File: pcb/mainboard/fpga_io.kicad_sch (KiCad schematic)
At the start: 18 parts, among them SW3 DSHP02TS, U3 XC7Z010-CLG400

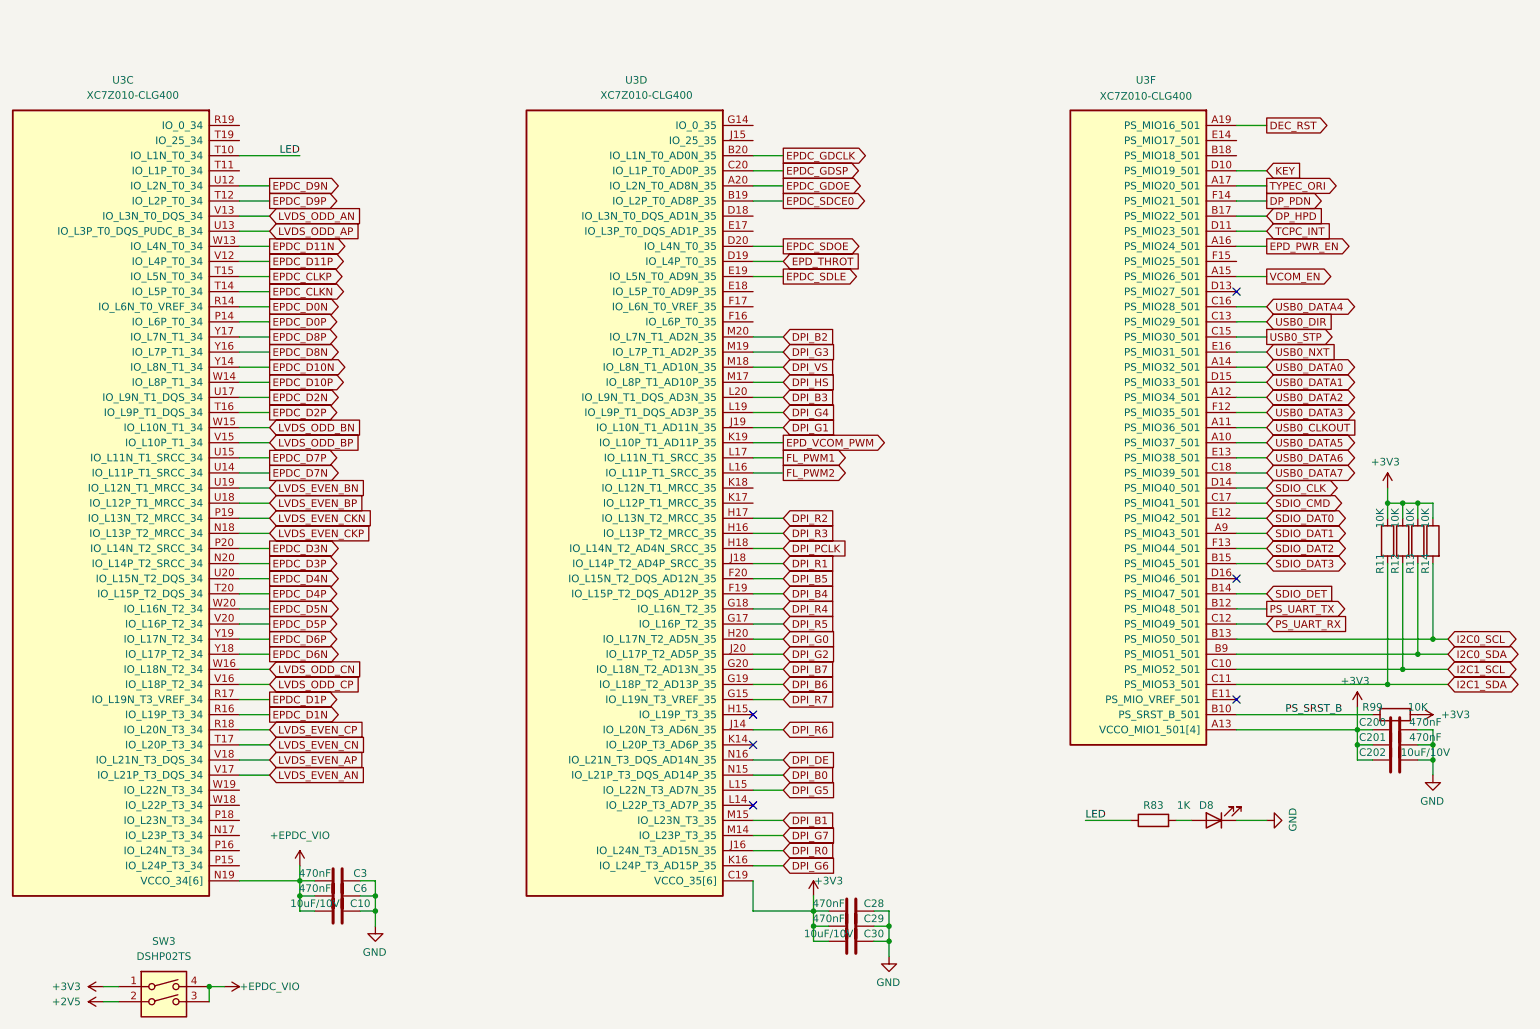
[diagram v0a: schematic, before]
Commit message: PCB r0p10 wip
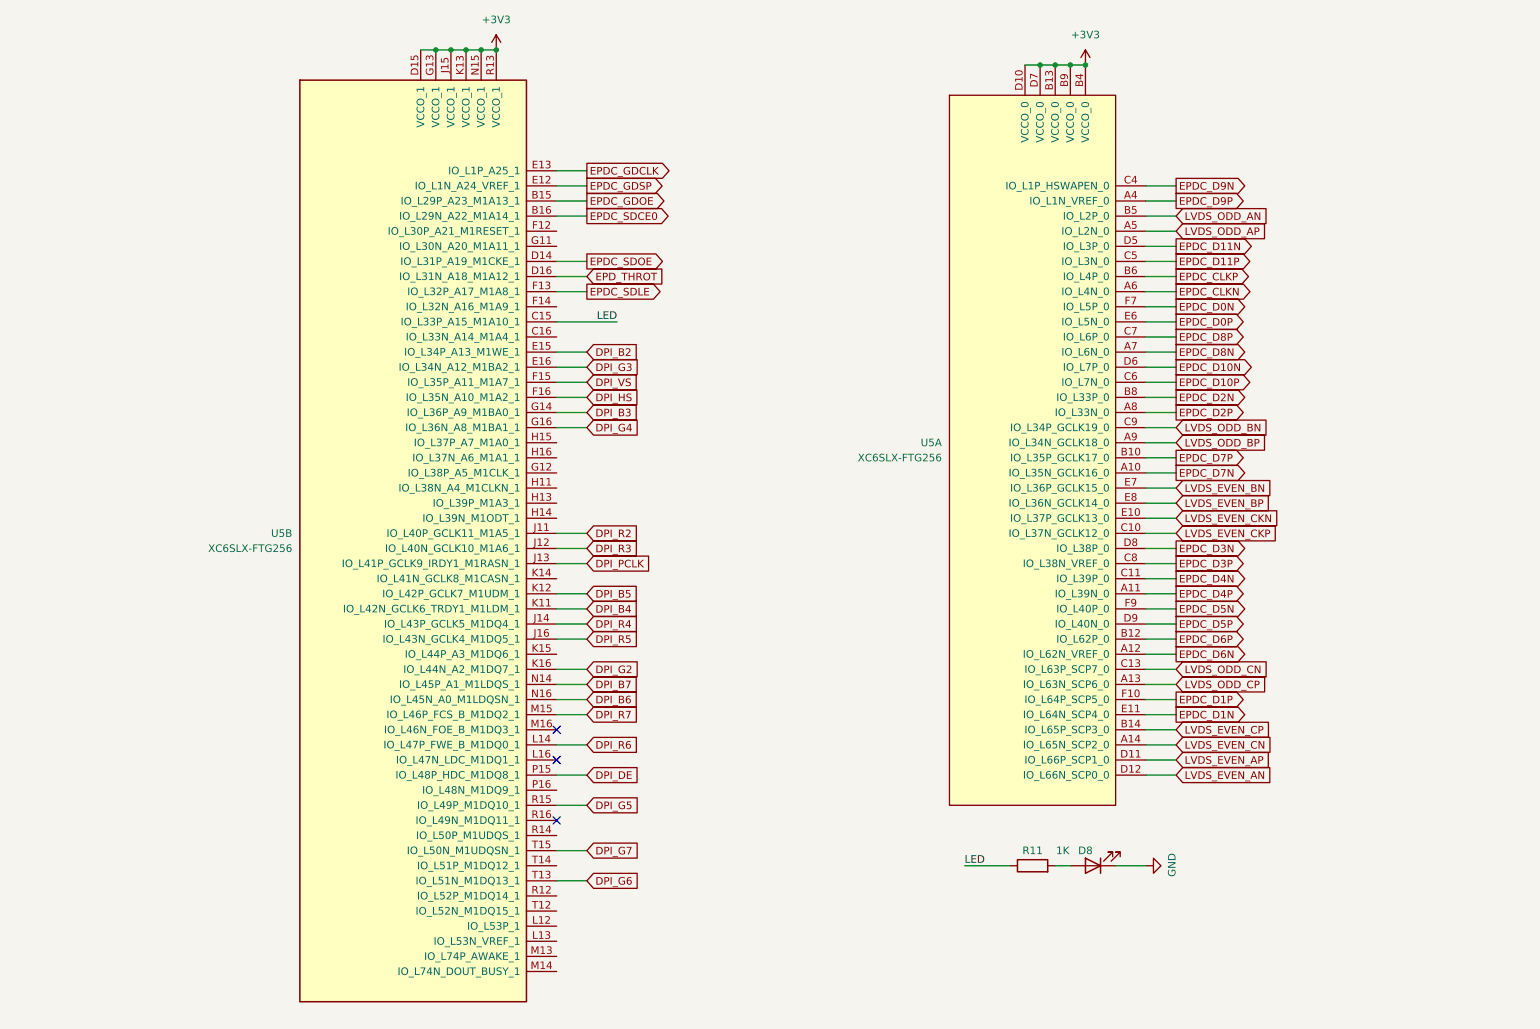
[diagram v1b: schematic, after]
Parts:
- removed C10, C202, C30: 10uF/10V, Capacitor_SMD:C_0603_1608Metric, symbol Device:C
- removed C200, C201, C28, C29, C3, C6: 470nF, Capacitor_SMD:C_0402_1005Metric, symbol Device:C
- removed R12, R13, R14, R99: 10K, Resistor_SMD:R_0402_1005Metric, symbol Device:R
- removed R83: 1K, Resistor_SMD:R_0402_1005Metric, symbol Device:R
- removed SW3: DSHP02TS, Button_Switch_SMD:SW_DIP_SPSTx02_Slide_KingTek_DSHP02TS_W7.62mm_P1.27mm, symbol Switch:SW_DIP_x02
- removed U3: XC7Z010-CLG400, Package_BGA:Xilinx_CLG400, symbol symbols:XC7Z007S-CLG400
- added U5: XC6SLX-FTG256, symbol symbols:XC6SLX-FTG256
- R11: value 10K -> 1K
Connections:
- net I2C1_SDA is gone; now on an unnamed net: R11.2
- net +3V3: now also U5.B13 (VCCO_0), U5.B4 (VCCO_0), U5.B9 (VCCO_0), U5.D10 (VCCO_0), U5.D15 (VCCO_1), U5.D7 (VCCO_0), U5.G13 (VCCO_1), U5.J15 (VCCO_1), U5.K13 (VCCO_1), U5.N15 (VCCO_1), U5.R13 (VCCO_1); no longer R11.1
- net DPI_B2: now also U5.E15 (IO_L34P_A13_M1WE_1)
- net DPI_B3: now also U5.G14 (IO_L36P_A9_M1BA0_1)
- net DPI_B4: now also U5.K11 (IO_L42N_GCLK6_TRDY1_M1LDM_1)
- net DPI_B5: now also U5.K12 (IO_L42P_GCLK7_M1UDM_1)
- net DPI_B6: now also U5.N16 (IO_L45N_A0_M1LDQSN_1)
- net DPI_B7: now also U5.N14 (IO_L45P_A1_M1LDQS_1)
- net DPI_DE: now also U5.P15 (IO_L48P_HDC_M1DQ8_1)
- net DPI_G2: now also U5.K16 (IO_L44N_A2_M1DQ7_1)
- net DPI_G3: now also U5.E16 (IO_L34N_A12_M1BA2_1)
- net DPI_G4: now also U5.G16 (IO_L36N_A8_M1BA1_1)
- net DPI_G5: now also U5.R15 (IO_L49P_M1DQ10_1)
- net DPI_G6: now also U5.T13 (IO_L51N_M1DQ13_1)
- net DPI_G7: now also U5.T15 (IO_L50N_M1UDQSN_1)
- net DPI_HS: now also U5.F16 (IO_L35N_A10_M1A2_1)
- net DPI_PCLK: now also U5.J13 (IO_L41P_GCLK9_IRDY1_M1RASN_1)
- net DPI_R2: now also U5.J11 (IO_L40P_GCLK11_M1A5_1)
- net DPI_R3: now also U5.J12 (IO_L40N_GCLK10_M1A6_1)
- net DPI_R4: now also U5.J14 (IO_L43P_GCLK5_M1DQ4_1)
- net DPI_R5: now also U5.J16 (IO_L43N_GCLK4_M1DQ5_1)
- net DPI_R6: now also U5.L14 (IO_L47P_FWE_B_M1DQ0_1)
- net DPI_R7: now also U5.M15 (IO_L46P_FCS_B_M1DQ2_1)
- net DPI_VS: now also U5.F15 (IO_L35P_A11_M1A7_1)
- net EPDC_CLKN: now also U5.A6 (IO_L4N_0)
- net EPDC_CLKP: now also U5.B6 (IO_L4P_0)
- net EPDC_D0N: now also U5.F7 (IO_L5P_0)
- net EPDC_D0P: now also U5.E6 (IO_L5N_0)
- net EPDC_D10N: now also U5.D6 (IO_L7P_0)
- net EPDC_D10P: now also U5.C6 (IO_L7N_0)
- net EPDC_D11N: now also U5.D5 (IO_L3P_0)
- net EPDC_D11P: now also U5.C5 (IO_L3N_0)
- net EPDC_D1N: now also U5.E11 (IO_L64N_SCP4_0)
- net EPDC_D1P: now also U5.F10 (IO_L64P_SCP5_0)
- net EPDC_D2N: now also U5.B8 (IO_L33P_0)
- net EPDC_D2P: now also U5.A8 (IO_L33N_0)
- net EPDC_D3N: now also U5.D8 (IO_L38P_0)
- net EPDC_D3P: now also U5.C8 (IO_L38N_VREF_0)
- net EPDC_D4N: now also U5.C11 (IO_L39P_0)
- net EPDC_D4P: now also U5.A11 (IO_L39N_0)
- net EPDC_D5N: now also U5.F9 (IO_L40P_0)
- net EPDC_D5P: now also U5.D9 (IO_L40N_0)
- net EPDC_D6N: now also U5.A12 (IO_L62N_VREF_0)
- net EPDC_D6P: now also U5.B12 (IO_L62P_0)
- net EPDC_D7N: now also U5.A10 (IO_L35N_GCLK16_0)
- net EPDC_D7P: now also U5.B10 (IO_L35P_GCLK17_0)
- net EPDC_D8N: now also U5.A7 (IO_L6N_0)
- net EPDC_D8P: now also U5.C7 (IO_L6P_0)
- net EPDC_D9N: now also U5.C4 (IO_L1P_HSWAPEN_0)
- net EPDC_D9P: now also U5.A4 (IO_L1N_VREF_0)
- net EPDC_GDCLK: now also U5.E13 (IO_L1P_A25_1)
- net EPDC_GDOE: now also U5.B15 (IO_L29P_A23_M1A13_1)
- net EPDC_GDSP: now also U5.E12 (IO_L1N_A24_VREF_1)
- net EPDC_SDCE0: now also U5.B16 (IO_L29N_A22_M1A14_1)
- net EPDC_SDLE: now also U5.F13 (IO_L32P_A17_M1A8_1)
- net EPDC_SDOE: now also U5.D14 (IO_L31P_A19_M1CKE_1)
- net EPD_THROT: now also U5.D16 (IO_L31N_A18_M1A12_1)
- net LED: now also R11.1, U5.C15 (IO_L33P_A15_M1A10_1)
- net LVDS_EVEN_AN: now also U5.D12 (IO_L66N_SCP0_0)
- net LVDS_EVEN_AP: now also U5.D11 (IO_L66P_SCP1_0)
- net LVDS_EVEN_BN: now also U5.E7 (IO_L36P_GCLK15_0)
- net LVDS_EVEN_BP: now also U5.E8 (IO_L36N_GCLK14_0)
- net LVDS_EVEN_CKN: now also U5.E10 (IO_L37P_GCLK13_0)
- net LVDS_EVEN_CKP: now also U5.C10 (IO_L37N_GCLK12_0)
- net LVDS_EVEN_CN: now also U5.A14 (IO_L65N_SCP2_0)
- net LVDS_EVEN_CP: now also U5.B14 (IO_L65P_SCP3_0)
- net LVDS_ODD_AN: now also U5.B5 (IO_L2P_0)
- net LVDS_ODD_AP: now also U5.A5 (IO_L2N_0)
- net LVDS_ODD_BN: now also U5.C9 (IO_L34P_GCLK19_0)
- net LVDS_ODD_BP: now also U5.A9 (IO_L34N_GCLK18_0)
- net LVDS_ODD_CN: now also U5.C13 (IO_L63P_SCP7_0)
- net LVDS_ODD_CP: now also U5.A13 (IO_L63N_SCP6_0)
- no-connect marks 6 -> 3

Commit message: PCB r0p10
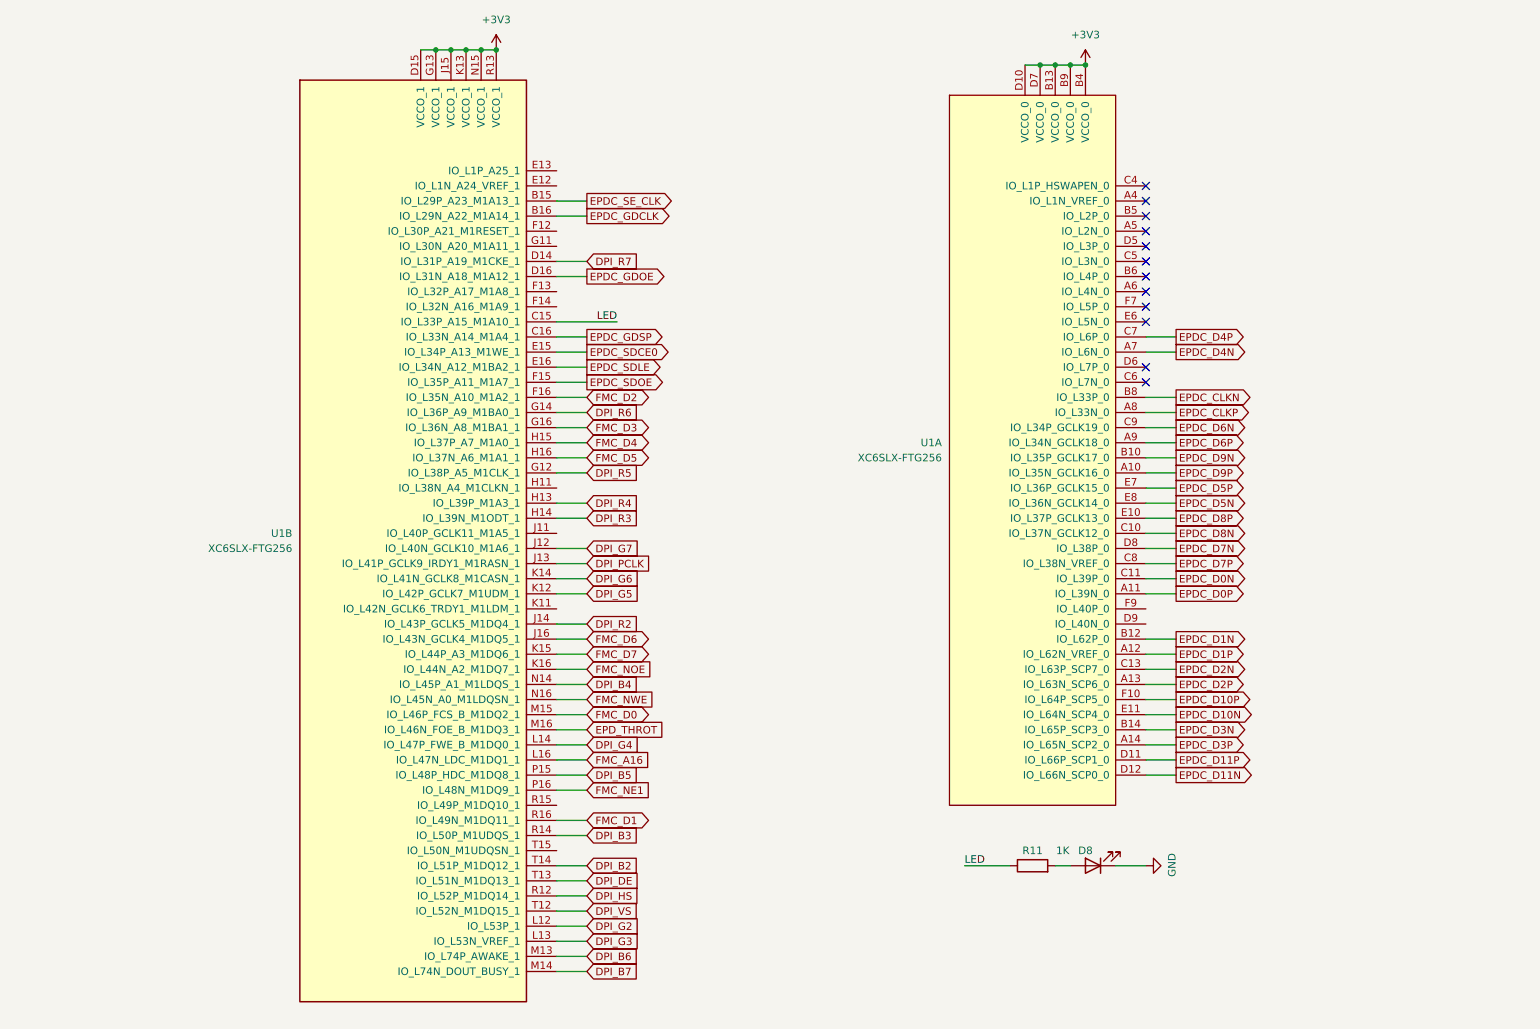
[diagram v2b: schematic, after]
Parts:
- U1: renamed from U5; footprint (none) -> footprints:Xilinx_FTG256
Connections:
- net LVDS_EVEN_AN is gone; now on net EPDC_D11N: U1.D12 (IO_L66N_SCP0_0)
- net LVDS_EVEN_AP is gone; now on net EPDC_D11P: U1.D11 (IO_L66P_SCP1_0)
- net LVDS_EVEN_BN is gone; now on net EPDC_D5P: U1.E7 (IO_L36P_GCLK15_0)
- net LVDS_EVEN_BP is gone; now on net EPDC_D5N: U1.E8 (IO_L36N_GCLK14_0)
- net LVDS_EVEN_CKN is gone; now on net EPDC_D8P: U1.E10 (IO_L37P_GCLK13_0)
- net LVDS_EVEN_CKP is gone; now on net EPDC_D8N: U1.C10 (IO_L37N_GCLK12_0)
- net LVDS_EVEN_CN is gone; now on net EPDC_D3P: U1.A14 (IO_L65N_SCP2_0)
- net LVDS_EVEN_CP is gone; now on net EPDC_D3N: U1.B14 (IO_L65P_SCP3_0)
- net LVDS_ODD_BN is gone; now on net EPDC_D6N: U1.C9 (IO_L34P_GCLK19_0)
- net LVDS_ODD_BP is gone; now on net EPDC_D6P: U1.A9 (IO_L34N_GCLK18_0)
- net LVDS_ODD_CN is gone; now on net EPDC_D2N: U1.C13 (IO_L63P_SCP7_0)
- net LVDS_ODD_CP is gone; now on net EPDC_D2P: U1.A13 (IO_L63N_SCP6_0)
- net DPI_B2: now also U1.T14 (IO_L51P_M1DQ12_1); no longer U1.E15 (IO_L34P_A13_M1WE_1)
- net DPI_B3: now also U1.R14 (IO_L50P_M1UDQS_1); no longer U1.G14 (IO_L36P_A9_M1BA0_1)
- net DPI_B4: now also U1.N14 (IO_L45P_A1_M1LDQS_1); no longer U1.K11 (IO_L42N_GCLK6_TRDY1_M1LDM_1)
- net DPI_B5: now also U1.P15 (IO_L48P_HDC_M1DQ8_1); no longer U1.K12 (IO_L42P_GCLK7_M1UDM_1)
- net DPI_B6: now also U1.M13 (IO_L74P_AWAKE_1); no longer U1.N16 (IO_L45N_A0_M1LDQSN_1)
- net DPI_B7: now also U1.M14 (IO_L74N_DOUT_BUSY_1); no longer U1.N14 (IO_L45P_A1_M1LDQS_1)
- net DPI_DE: now also U1.T13 (IO_L51N_M1DQ13_1); no longer U1.P15 (IO_L48P_HDC_M1DQ8_1)
- net DPI_G2: now also U1.L12 (IO_L53P_1); no longer U1.K16 (IO_L44N_A2_M1DQ7_1)
- net DPI_G3: now also U1.L13 (IO_L53N_VREF_1); no longer U1.E16 (IO_L34N_A12_M1BA2_1)
- net DPI_G4: now also U1.L14 (IO_L47P_FWE_B_M1DQ0_1); no longer U1.G16 (IO_L36N_A8_M1BA1_1)
- net DPI_G5: now also U1.K12 (IO_L42P_GCLK7_M1UDM_1); no longer U1.R15 (IO_L49P_M1DQ10_1)
- net DPI_G6: now also U1.K14 (IO_L41N_GCLK8_M1CASN_1); no longer U1.T13 (IO_L51N_M1DQ13_1)
- net DPI_G7: now also U1.J12 (IO_L40N_GCLK10_M1A6_1); no longer U1.T15 (IO_L50N_M1UDQSN_1)
- net DPI_HS: now also U1.R12 (IO_L52P_M1DQ14_1); no longer U1.F16 (IO_L35N_A10_M1A2_1)
- net DPI_R2: now also U1.J14 (IO_L43P_GCLK5_M1DQ4_1); no longer U1.J11 (IO_L40P_GCLK11_M1A5_1)
- net DPI_R3: now also U1.H14 (IO_L39N_M1ODT_1); no longer U1.J12 (IO_L40N_GCLK10_M1A6_1)
- net DPI_R4: now also U1.H13 (IO_L39P_M1A3_1); no longer U1.J14 (IO_L43P_GCLK5_M1DQ4_1)
- net DPI_R5: now also U1.G12 (IO_L38P_A5_M1CLK_1); no longer U1.J16 (IO_L43N_GCLK4_M1DQ5_1)
- net DPI_R6: now also U1.G14 (IO_L36P_A9_M1BA0_1); no longer U1.L14 (IO_L47P_FWE_B_M1DQ0_1)
- net DPI_R7: now also U1.D14 (IO_L31P_A19_M1CKE_1); no longer U1.M15 (IO_L46P_FCS_B_M1DQ2_1)
- net DPI_VS: now also U1.T12 (IO_L52N_M1DQ15_1); no longer U1.F15 (IO_L35P_A11_M1A7_1)
- net EPDC_CLKN: now also U1.B8 (IO_L33P_0); no longer U1.A6 (IO_L4N_0)
- net EPDC_CLKP: now also U1.A8 (IO_L33N_0); no longer U1.B6 (IO_L4P_0)
- net EPDC_D0N: now also U1.C11 (IO_L39P_0); no longer U1.F7 (IO_L5P_0)
- net EPDC_D0P: now also U1.A11 (IO_L39N_0); no longer U1.E6 (IO_L5N_0)
- net EPDC_D10N: now also U1.E11 (IO_L64N_SCP4_0); no longer U1.D6 (IO_L7P_0)
- net EPDC_D10P: now also U1.F10 (IO_L64P_SCP5_0); no longer U1.C6 (IO_L7N_0)
- net EPDC_D11N: no longer U1.D5 (IO_L3P_0)
- net EPDC_D11P: no longer U1.C5 (IO_L3N_0)
- net EPDC_D1N: now also U1.B12 (IO_L62P_0); no longer U1.E11 (IO_L64N_SCP4_0)
- net EPDC_D1P: now also U1.A12 (IO_L62N_VREF_0); no longer U1.F10 (IO_L64P_SCP5_0)
- net EPDC_D2N: no longer U1.B8 (IO_L33P_0)
- net EPDC_D2P: no longer U1.A8 (IO_L33N_0)
- net EPDC_D3N: no longer U1.D8 (IO_L38P_0)
- net EPDC_D3P: no longer U1.C8 (IO_L38N_VREF_0)
- net EPDC_D4N: now also U1.A7 (IO_L6N_0); no longer U1.C11 (IO_L39P_0)
- net EPDC_D4P: now also U1.C7 (IO_L6P_0); no longer U1.A11 (IO_L39N_0)
- net EPDC_D5N: no longer U1.F9 (IO_L40P_0)
- net EPDC_D5P: no longer U1.D9 (IO_L40N_0)
- net EPDC_D6N: no longer U1.A12 (IO_L62N_VREF_0)
- net EPDC_D6P: no longer U1.B12 (IO_L62P_0)
- net EPDC_D7N: now also U1.D8 (IO_L38P_0); no longer U1.A10 (IO_L35N_GCLK16_0)
- net EPDC_D7P: now also U1.C8 (IO_L38N_VREF_0); no longer U1.B10 (IO_L35P_GCLK17_0)
- net EPDC_D8N: no longer U1.A7 (IO_L6N_0)
- net EPDC_D8P: no longer U1.C7 (IO_L6P_0)
- net EPDC_D9N: now also U1.B10 (IO_L35P_GCLK17_0); no longer U1.C4 (IO_L1P_HSWAPEN_0)
- net EPDC_D9P: now also U1.A10 (IO_L35N_GCLK16_0); no longer U1.A4 (IO_L1N_VREF_0)
- net EPDC_GDCLK: now also U1.B16 (IO_L29N_A22_M1A14_1); no longer U1.E13 (IO_L1P_A25_1)
- net EPDC_GDOE: now also U1.D16 (IO_L31N_A18_M1A12_1); no longer U1.B15 (IO_L29P_A23_M1A13_1)
- net EPDC_GDSP: now also U1.C16 (IO_L33N_A14_M1A4_1); no longer U1.E12 (IO_L1N_A24_VREF_1)
- net EPDC_SDCE0: now also U1.E15 (IO_L34P_A13_M1WE_1); no longer U1.B16 (IO_L29N_A22_M1A14_1)
- net EPDC_SDLE: now also U1.E16 (IO_L34N_A12_M1BA2_1); no longer U1.F13 (IO_L32P_A17_M1A8_1)
- net EPDC_SDOE: now also U1.F15 (IO_L35P_A11_M1A7_1); no longer U1.D14 (IO_L31P_A19_M1CKE_1)
- net EPD_THROT: now also U1.M16 (IO_L46N_FOE_B_M1DQ3_1); no longer U1.D16 (IO_L31N_A18_M1A12_1)
- net FMC_D4: now reaches U1.H15 (IO_L37P_A7_M1A0_1)
- net FMC_D5: now reaches U1.H16 (IO_L37N_A6_M1A1_1)
- net FMC_D7: now reaches U1.K15 (IO_L44P_A3_M1DQ6_1)
- net FMC_A16: now reaches U1.L16 (IO_L47N_LDC_M1DQ1_1)
- net FMC_NE1: now reaches U1.P16 (IO_L48N_M1DQ9_1)
- net FMC_D1: now reaches U1.R16 (IO_L49N_M1DQ11_1)
- net LVDS_ODD_AN: no longer names the net of U1.B5 (IO_L2P_0)
- net LVDS_ODD_AP: no longer names the net of U1.A5 (IO_L2N_0)
- new net EPDC_SE_CLK: U1.B15 (IO_L29P_A23_M1A13_1)
- new net FMC_D0: U1.M15 (IO_L46P_FCS_B_M1DQ2_1)
- new net FMC_D2: U1.F16 (IO_L35N_A10_M1A2_1)
- new net FMC_D3: U1.G16 (IO_L36N_A8_M1BA1_1)
- new net FMC_D6: U1.J16 (IO_L43N_GCLK4_M1DQ5_1)
- new net FMC_NOE: U1.K16 (IO_L44N_A2_M1DQ7_1)
- new net FMC_NWE: U1.N16 (IO_L45N_A0_M1LDQSN_1)
- no-connect marks 3 -> 12
